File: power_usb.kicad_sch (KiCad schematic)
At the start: 5 parts, among them J3 USB_C_Receptacle_USB2.0_16P, U10 USBLC6-2SC6

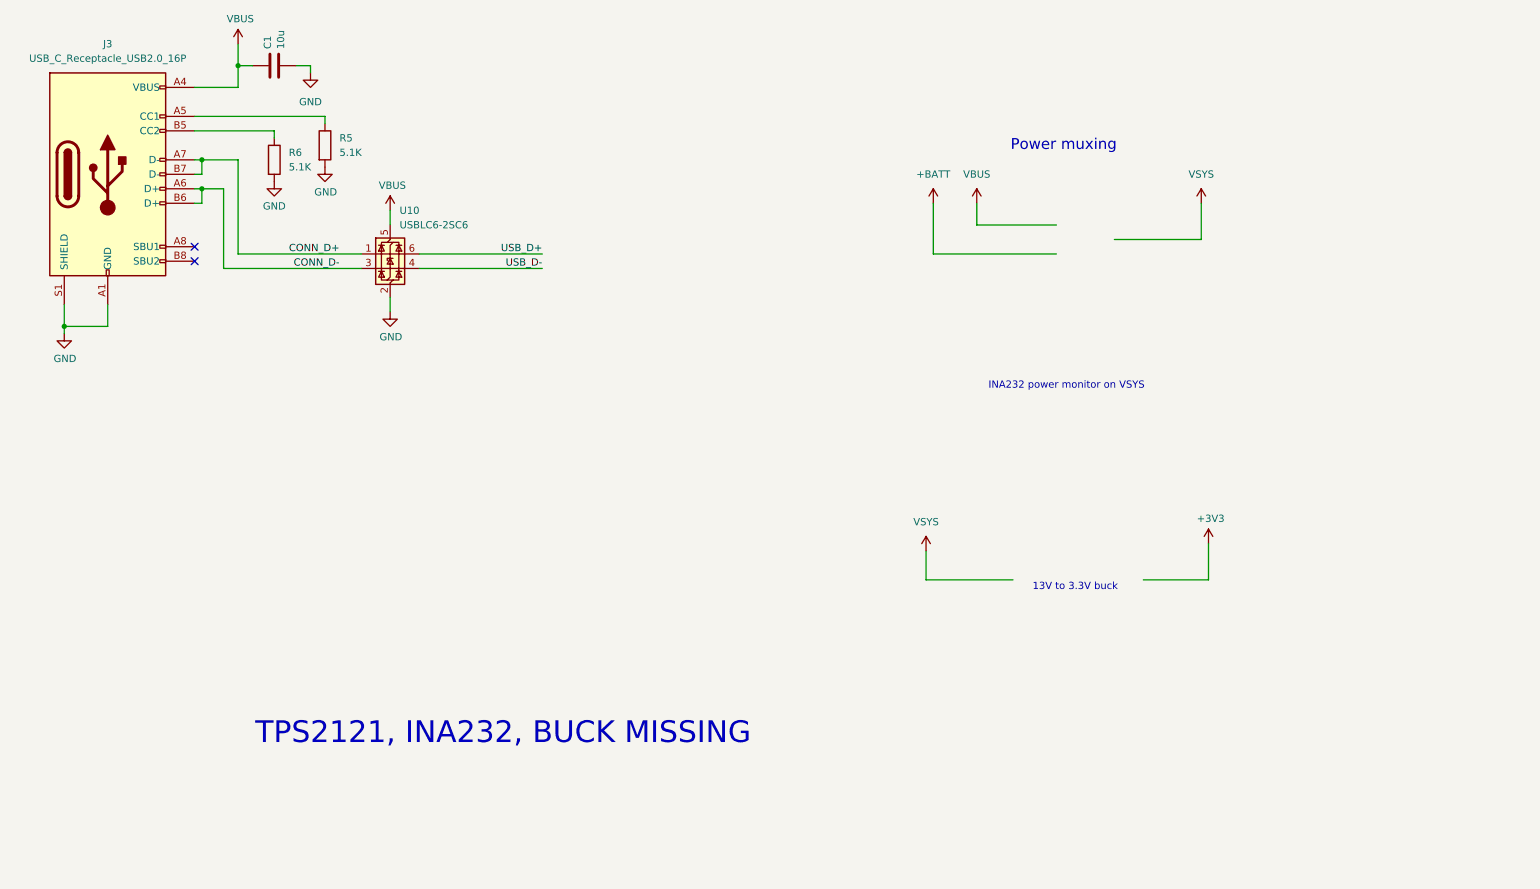
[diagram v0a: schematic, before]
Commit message: progress, particularly on power
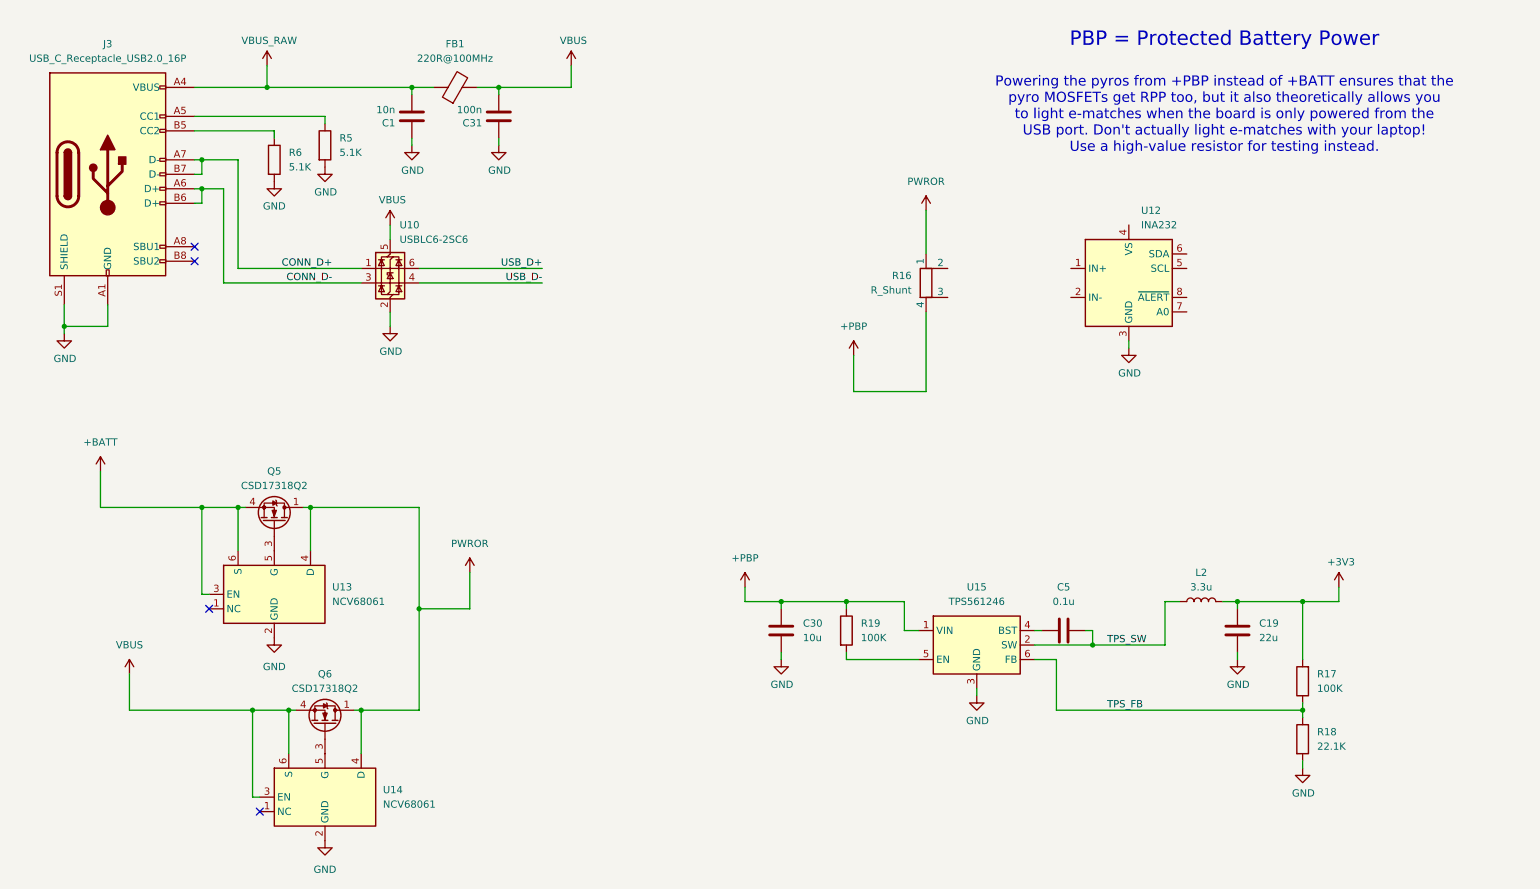
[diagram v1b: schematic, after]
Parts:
- added C19: 22u, Capacitor_SMD:C_0805_2012Metric, symbol Device:C
- added C30: 10u, Capacitor_SMD:C_0805_2012Metric, symbol Device:C
- added C31: 100n, Capacitor_SMD:C_0603_1608Metric, symbol Device:C
- added C5: 0.1u, Capacitor_SMD:C_0603_1608Metric, symbol Device:C
- added FB1: 220R@100MHz, Inductor_SMD:L_0603_1608Metric, symbol Device:FerriteBead
- added L2: 3.3u, symbol Device:L
- added Q5, Q6: CSD17318Q2, Package_SON:Texas_DQK, symbol Transistor_FET:CSD17313Q2
- added R16: R_Shunt, Resistor_SMD:R_Shunt_Vishay_WSKW0612, symbol Device:R_Shunt
- added R17, R19: 100K, Resistor_SMD:R_0603_1608Metric, symbol Device:R
- added R18: 22.1K, Resistor_SMD:R_0603_1608Metric, symbol Device:R
- added U12: INA232, LRI_partlib:TSOT-23-8, symbol LRI_partlib:INA232
- added U13, U14: NCV68061, Package_TO_SOT_SMD:SOT-23-6, symbol LRI_partlib:NCV68061
- added U15: TPS561246, Package_TO_SOT_SMD:SOT-563, symbol LRI_partlib:TPS561246
- C1: value 10u -> 10n; footprint Capacitor_SMD:C_0805_2012Metric -> Capacitor_SMD:C_0603_1608Metric
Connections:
- net +3V3: now also C19.1, L2.2, R17.2
- net +BATT: now also Q5.4 (S), Q5.7 (S), U13.3 (EN), U13.6 (S)
- net GND: now also C1.1, C19.2, C30.2, C31.1, R18.2, U12.3 (GND), U13.2 (GND), U14.2 (GND), U15.3 (GND); no longer C1.2
- net VBUS: now also C31.2, FB1.2, Q6.4 (S), Q6.7 (S), U14.3 (EN), U14.6 (S); no longer C1.1, J3.A4 (VBUS), J3.A9 (VBUS), J3.B4 (VBUS), J3.B9 (VBUS)
- new net: C5.1, U15.4 (BST)
- new net: R19.2, U15.5 (EN)
- new net: Q5.3 (G), U13.5 (G)
- new net: Q6.3 (G), U14.5 (G)
- new net +PBP: C30.1, R16.4, R19.1, U15.1 (VIN)
- new net PWROR: Q5.1 (D), Q5.2 (D), Q5.5 (D), Q5.6 (D), Q5.8 (D), Q6.1 (D), Q6.2 (D), Q6.5 (D), Q6.6 (D), Q6.8 (D), R16.1, U13.4 (D), U14.4 (D)
- new net TPS_FB: R17.1, R18.1, U15.6 (FB)
- new net TPS_SW: C5.2, L2.1, U15.2 (SW)
- new net VBUS_RAW: C1.2, FB1.1, J3.A4 (VBUS), J3.A9 (VBUS), J3.B4 (VBUS), J3.B9 (VBUS)
- no-connect marks 2 -> 4
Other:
- note added: "PBP = Protected Battery Power"
- note added: "Powering the pyros from +PBP instead of +BATT ensures that the pyro MOSFETs get RPP too, but it also theoretically allows you to light e-matches when the board is only powered from the USB port. Don't actually light e-matches with your laptop! Use a high-value resistor for testing instead."
- note removed: "13V to 3.3V buck"
- note removed: "INA232 power monitor on VSYS"
- note removed: "Power muxing"
- note removed: "TPS2121, INA232, BUCK MISSING"
- moved on the sheet: C1, U10
